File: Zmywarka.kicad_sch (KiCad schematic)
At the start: 69 parts, among them J1 Conn_01x08, Q1 BC817, Q2 BC817, Q3 BC817, Q4 BC817, SW1 SW_MEC_5G, SW2 SW_MEC_5G, SW3 SW_MEC_5G, SW4 SW_MEC_5G, U1 74HC595, U2 74HC595

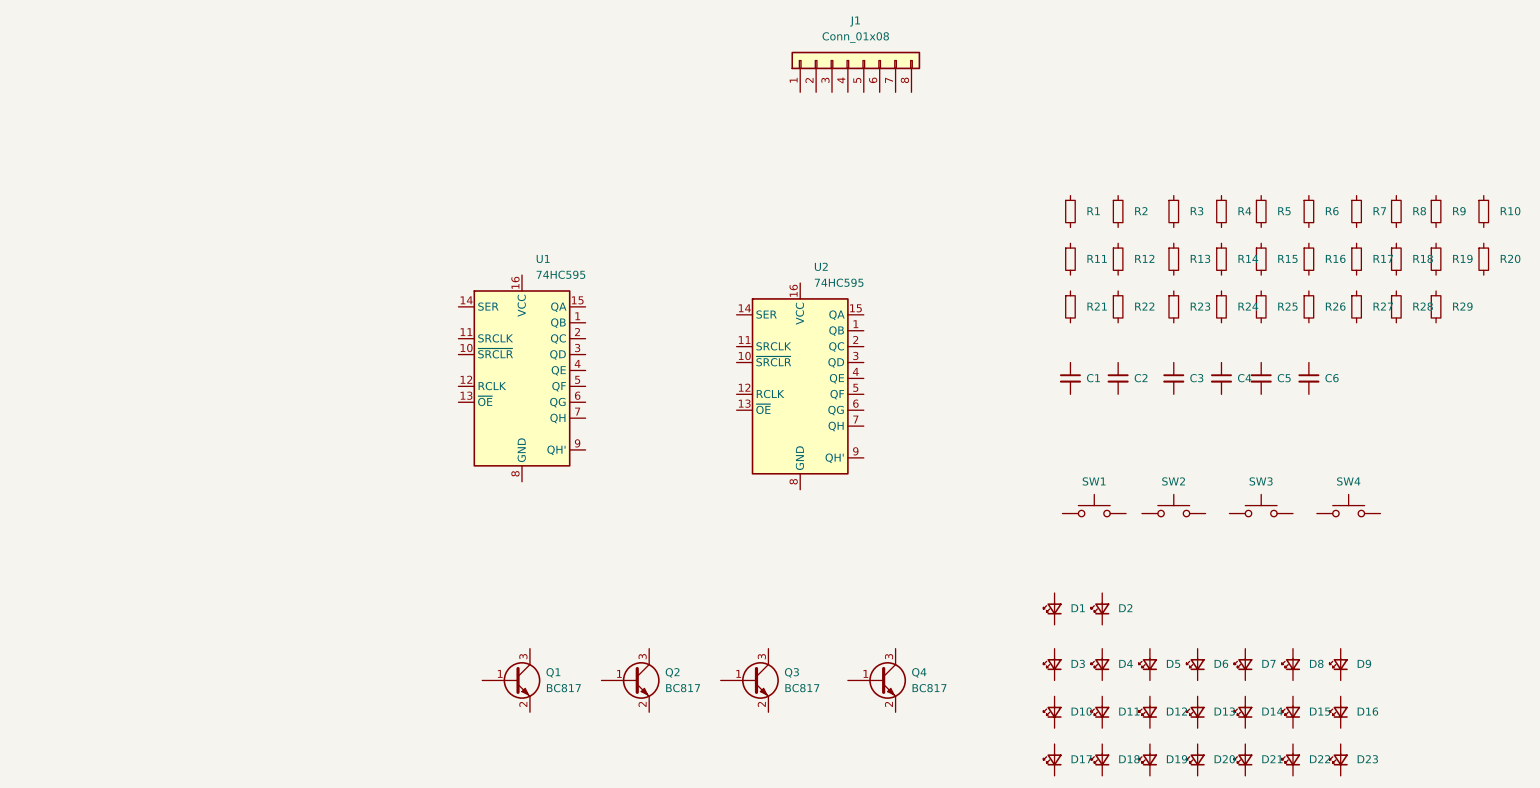
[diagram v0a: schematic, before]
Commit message: edit
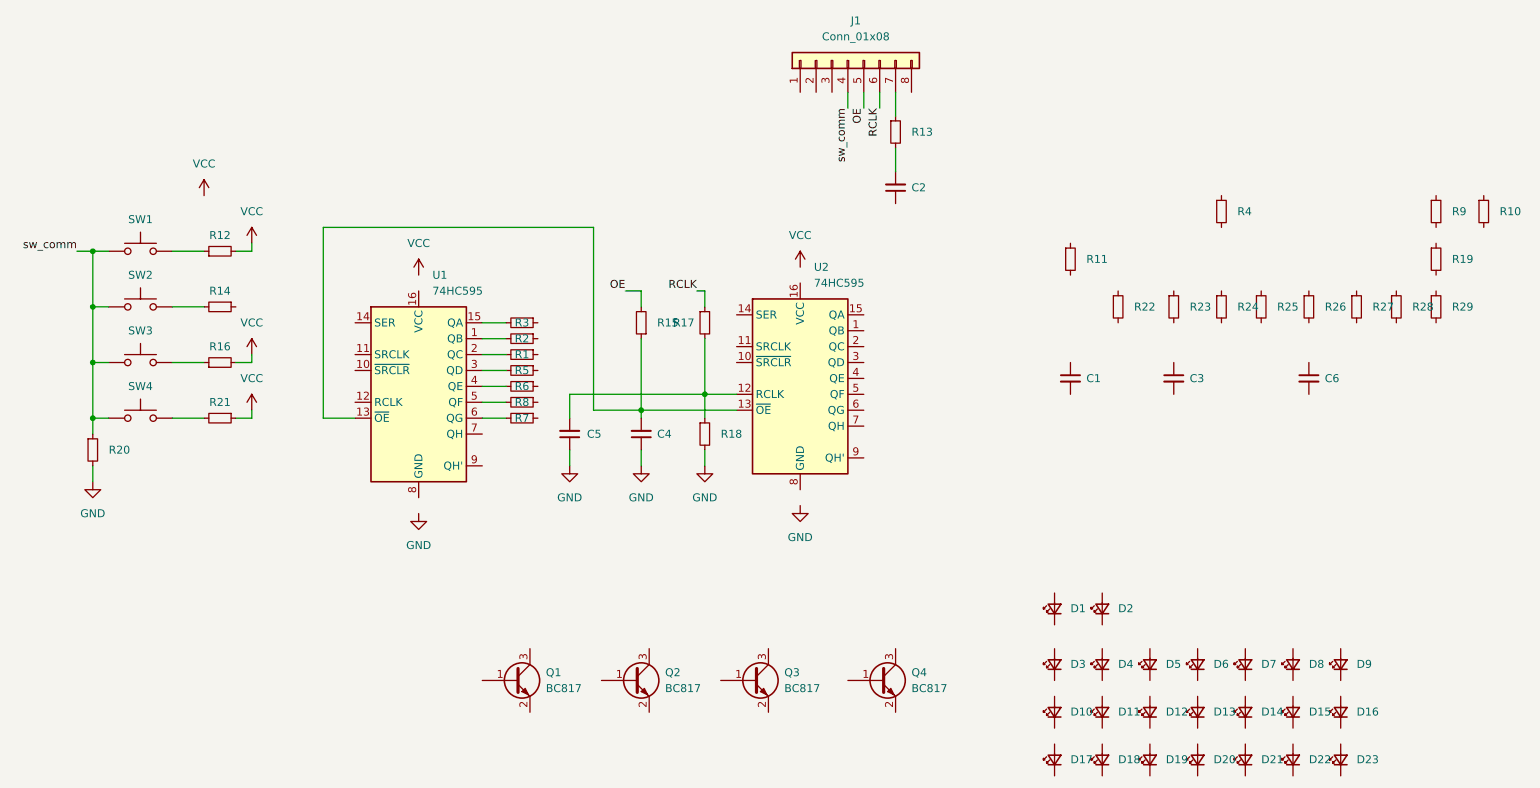
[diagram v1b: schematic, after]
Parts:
- removed SW1, SW2, SW3, SW4: SW_MEC_5G, Button_Switch_SMD:SW_Push_1P1T_NO_6x6mm_H9.5mm, symbol Switch:SW_MEC_5G
- added SW1, SW2, SW3, SW4: SW_Omron_B3FS, Button_Switch_SMD:SW_Push_1P1T_NO_6x6mm_H9.5mm, symbol Switch:SW_Omron_B3FS
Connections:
- net at U2.12 (RCLK): now also C5.2, R17.2, R18.1
- net at U2.13 (~{OE}): now also C4.2, R15.1, U1.13 (~{OE})
- net OE: now reaches R15.2
- net OE: now also J1.5 (Pin_5)
- net VCC: now reaches R21.1
- net VCC: now also R12.2, R16.2
- net at R21.2: now also SW4.2
- net at R8.2: now also U1.5 (QF)
- net at R3.2: now also U1.15 (QA)
- net at R13.1: now also J1.7 (Pin_7)
- net at R13.2: now also C2.2
- net GND: now reaches C4.1
- net GND: now also C5.1, R18.2, R20.2
- net at R6.2: now also U1.4 (QE)
- net at R14.2: now also SW2.2
- net sw_comm: now reaches R20.1
- net sw_comm: now also J1.4 (Pin_4), SW1.1, SW2.1, SW3.1, SW4.1
- net at R1.2: now also U1.2 (QC)
- net at R7.2: now also U1.6 (QG)
- net at R5.2: now also U1.3 (QD)
- net RCLK: now reaches J1.6 (Pin_6)
- net RCLK: now also R17.1
- net at U1.1 (QB): now also R2.2
- net at R16.1: now also SW3.2
- net at R12.1: now also SW1.2
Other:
- moved on the sheet: C2, C4, C5, R1, R12, R13, R14, R15, R16, R17, R18, R2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
